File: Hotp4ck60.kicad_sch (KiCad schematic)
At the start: 46 parts, among them J1 HRO_TYPE-C-31-M-12, SW44 RST, U1 nRF52840, U2 SRV05-4, Y1 32 MHz, Y2 32.768 Khz

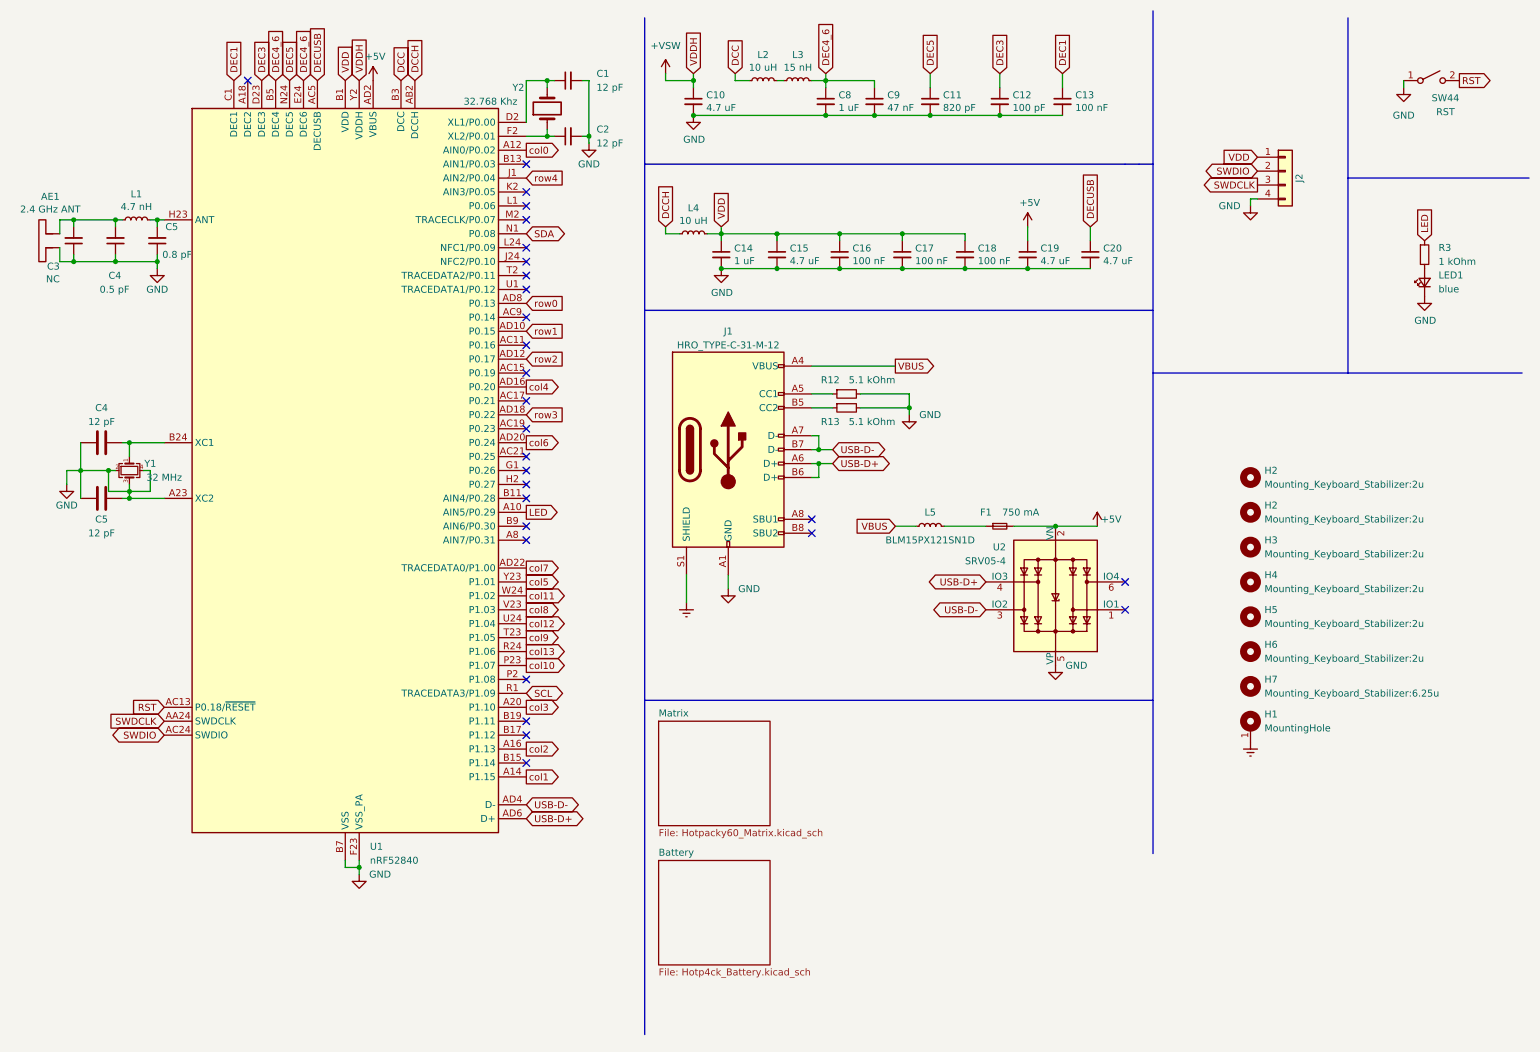
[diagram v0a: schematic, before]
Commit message: Fixed position & etc..
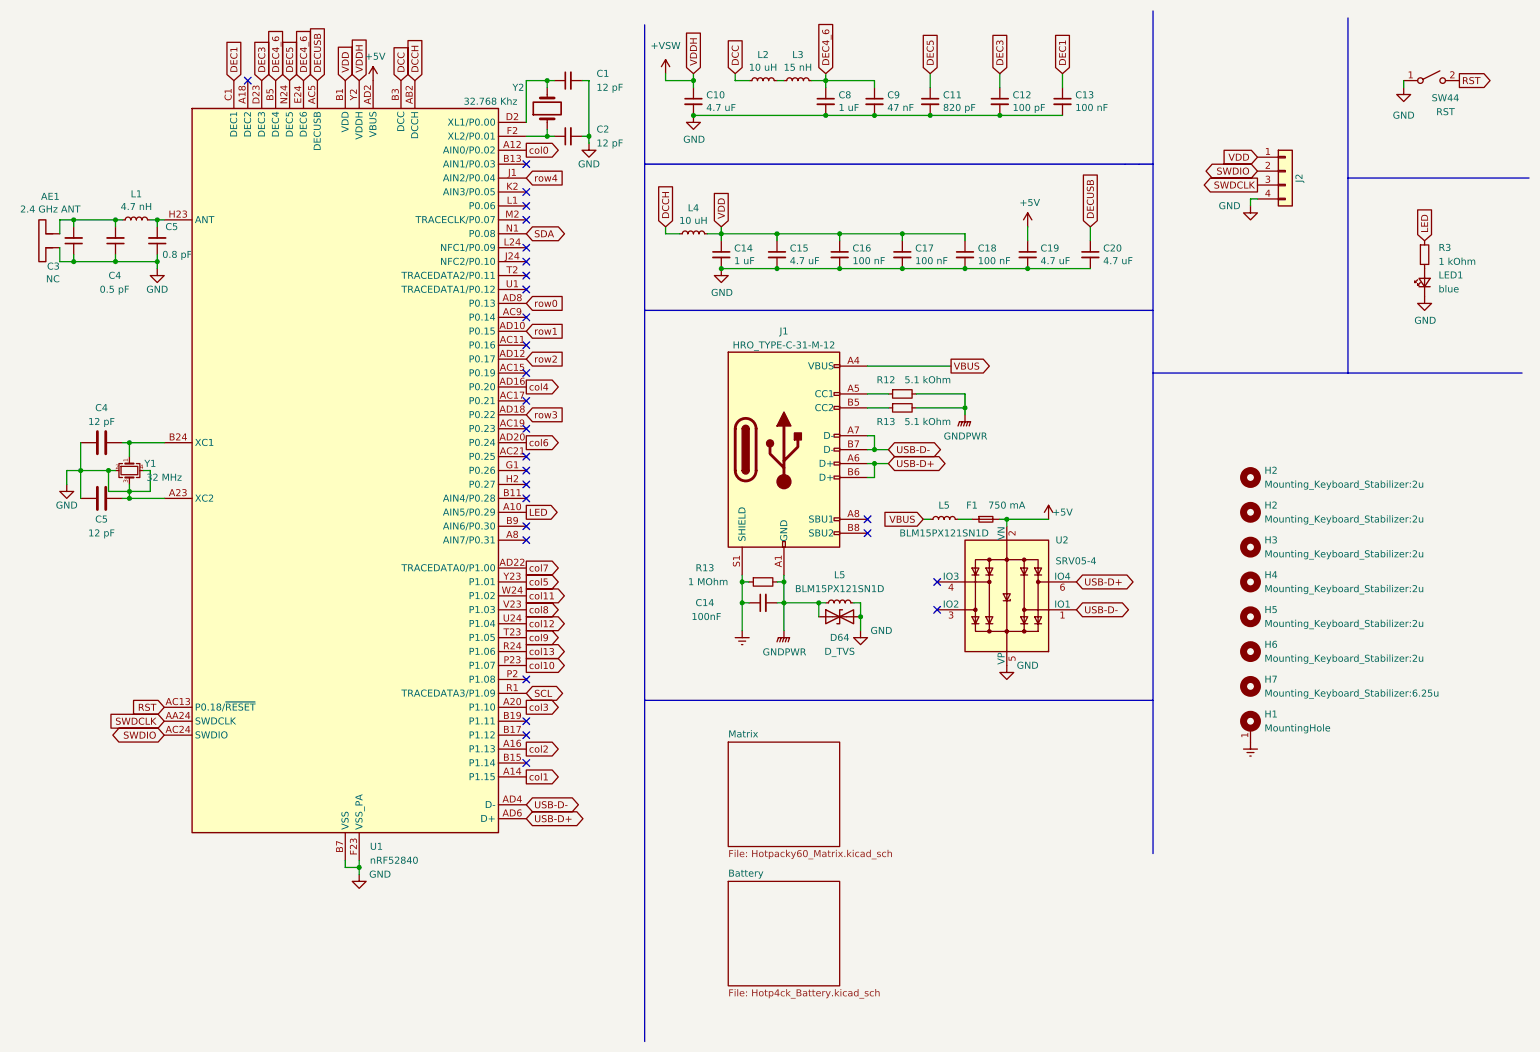
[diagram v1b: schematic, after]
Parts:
- added C14: 100nF, Capacitor_SMD:C_0402_1005Metric, symbol Device:C_Small
- added D64: D_TVS, Diode_SMD:D_SOD-123F, symbol Device:D_TVS
- added L5: BLM15PX121SN1D, Inductor_SMD:L_0402_1005Metric, symbol Device:L_Small
- added R13: 1 MOhm, Resistor_SMD:R_0402_1005Metric, symbol Device:R_Small
- LED1: footprint LED_SMD:LED_0402_1005Metric -> LED_SMD:LED_0603_1608Metric
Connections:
- net Earth: now also C14.1, R13.1
- net GND: now also D64.2 (A2), L5.1; no longer J1.A1 (GND), J1.A12 (GND), J1.B1 (GND), J1.B12 (GND), R12.2, R13.2
- net USB-D+: now also U2.6 (IO4); no longer U2.4 (IO3)
- net USB-D-: now also U2.1 (IO1); no longer U2.3 (IO2)
- new net GNDPWR: C14.2, D64.1 (A1), J1.A1 (GND), J1.A12 (GND), J1.B1 (GND), J1.B12 (GND), L5.2, R12.2, R13.2, R13.2
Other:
- moved on the sheet: F1, J1, L5, R12, R13, U2
